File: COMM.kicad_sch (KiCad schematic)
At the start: 6 parts, among them J2 USB_C_Receptacle_USB2.0, U2 CH340E

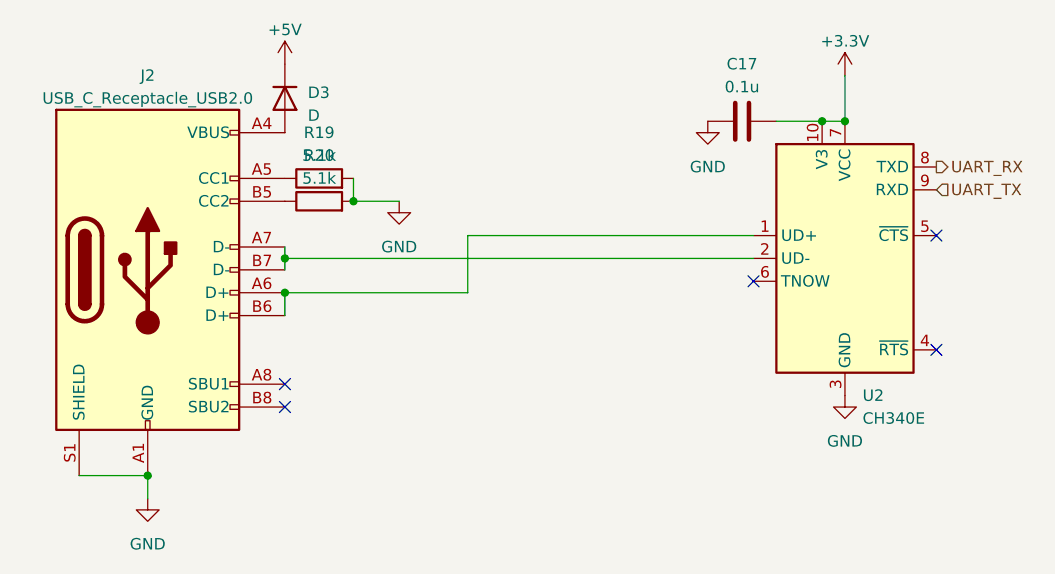
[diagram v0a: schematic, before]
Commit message: なにか変えた
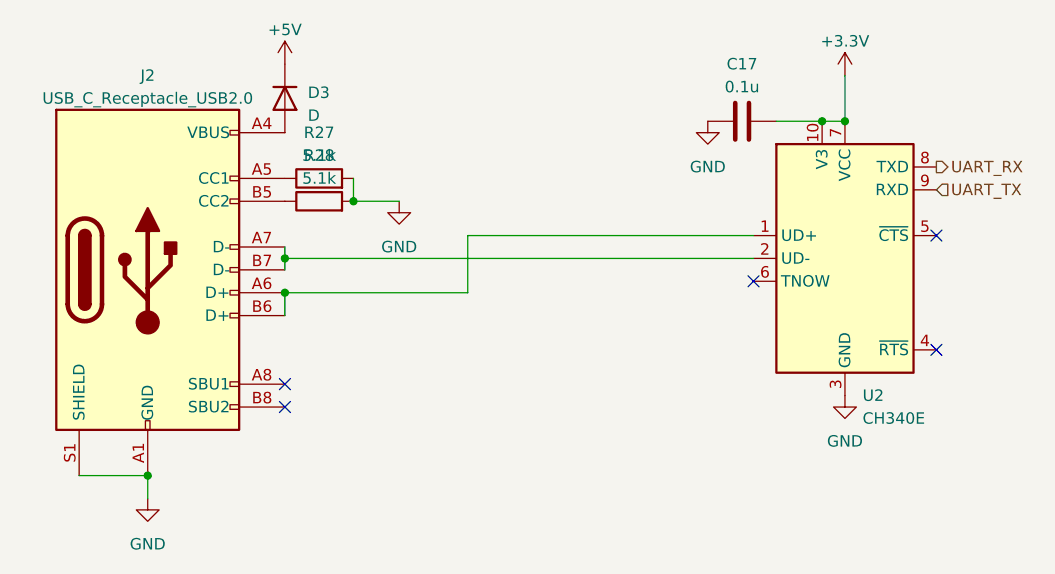
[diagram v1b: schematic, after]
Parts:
- renumbered R19 to R27, R20 to R28
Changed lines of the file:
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@@
         )
         (path "/01e9384d-acb3-40ee-83e0-c5c8a07f30ec/086dea9c-06af-4312-9d68-ae693603fcbc"
-          (reference "#PWR071") (unit 1)
+          (reference "#PWR079") (unit 1)
         )
       )
@@
   (symbol (lib_id "power:+5V") (at 119.38 59.69 0) (unit 1)
     (in_bom yes) (on_board yes) (dnp no) (fields_autoplaced)
-    (property "Reference" "#PWR068" (at 119.38 63.5 0)
+    (property "Reference" "#PWR076" (at 119.38 63.5 0)
       (effects (font (size 1.27 1.27)) hide)
     )
@@
       (project "sMDU"
         (path "/01e9384d-acb3-40ee-83e0-c5c8a07f30ec/086dea9c-06af-4312-9d68-ae693603fcbc"
-          (reference "#PWR068") (unit 1)
+          (reference "#PWR076") (unit 1)
         )
       )
@@
   (symbol (lib_id "Device:R") (at 123.19 72.39 90) (unit 1)
     (in_bom yes) (on_board yes) (dnp no) (fields_autoplaced)
-    (property "Reference" "R19" (at 123.19 67.31 90)
+    (property "Reference" "R27" (at 123.19 67.31 90)
       (effects (font (size 1.27 1.27)))
     )
@@
       (project "sMDU"
         (path "/01e9384d-acb3-40ee-83e0-c5c8a07f30ec/086dea9c-06af-4312-9d68-ae693603fcbc"
-          (reference "R19") (unit 1)
+          (reference "R27") (unit 1)
         )
       )
@@
   (symbol (lib_id "Device:R") (at 123.19 74.93 90) (unit 1)
     (in_bom yes) (on_board yes) (dnp no) (fields_autoplaced)
-    (property "Reference" "R20" (at 123.19 69.85 90)
+    (property "Reference" "R28" (at 123.19 69.85 90)
       (effects (font (size 1.27 1.27)))
     )
@@
       (project "sMDU"
         (path "/01e9384d-acb3-40ee-83e0-c5c8a07f30ec/086dea9c-06af-4312-9d68-ae693603fcbc"
-          (reference "R20") (unit 1)
+          (reference "R28") (unit 1)
         )
       )
@@
         )
         (path "/01e9384d-acb3-40ee-83e0-c5c8a07f30ec/086dea9c-06af-4312-9d68-ae693603fcbc"
-          (reference "#PWR070") (unit 1)
+          (reference "#PWR078") (unit 1)
         )
       )
@@
   (symbol (lib_id "power:GND") (at 132.08 74.93 0) (unit 1)
     (in_bom yes) (on_board yes) (dnp no) (fields_autoplaced)
-    (property "Reference" "#PWR069" (at 132.08 81.28 0)
+    (property "Reference" "#PWR077" (at 132.08 81.28 0)
       (effects (font (size 1.27 1.27)) hide)
     )
@@
       (project "sMDU"
         (path "/01e9384d-acb3-40ee-83e0-c5c8a07f30ec/086dea9c-06af-4312-9d68-ae693603fcbc"
-          (reference "#PWR069") (unit 1)
+          (reference "#PWR077") (unit 1)
         )
       )
@@
         )
         (path "/01e9384d-acb3-40ee-83e0-c5c8a07f30ec/086dea9c-06af-4312-9d68-ae693603fcbc"
-          (reference "#PWR072") (unit 1)
+          (reference "#PWR080") (unit 1)
         )
       )
@@
   (symbol (lib_id "power:GND") (at 104.14 107.95 0) (unit 1)
     (in_bom yes) (on_board yes) (dnp no) (fields_autoplaced)
-    (property "Reference" "#PWR067" (at 104.14 114.3 0)
+    (property "Reference" "#PWR075" (at 104.14 114.3 0)
       (effects (font (size 1.27 1.27)) hide)
     )
@@
       (project "sMDU"
         (path "/01e9384d-acb3-40ee-83e0-c5c8a07f30ec/086dea9c-06af-4312-9d68-ae693603fcbc"
-          (reference "#PWR067") (unit 1)
-        )
-      )
+          (reference "#PWR075") (unit 1)
+        )
+      )
